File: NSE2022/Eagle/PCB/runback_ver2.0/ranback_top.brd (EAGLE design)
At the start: 100 x 61.3 mm, 25 parts

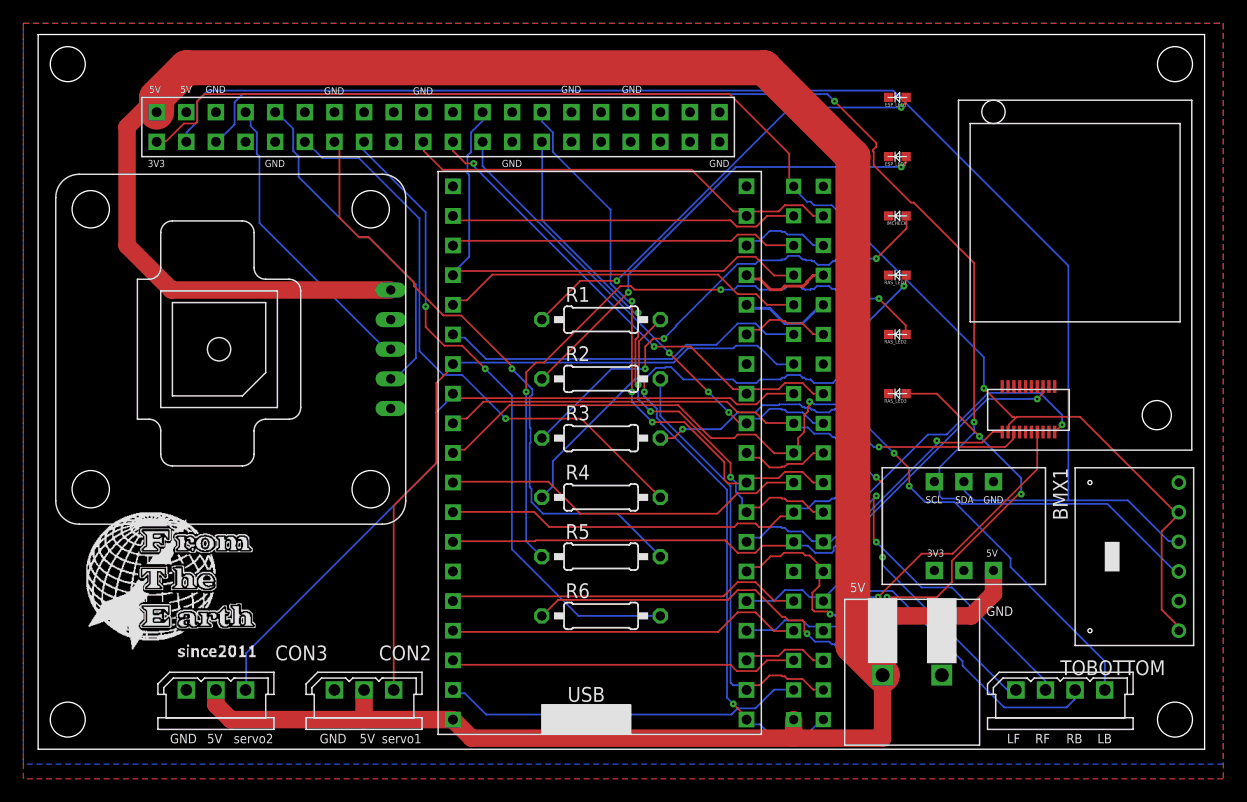
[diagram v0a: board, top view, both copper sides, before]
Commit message: sdf
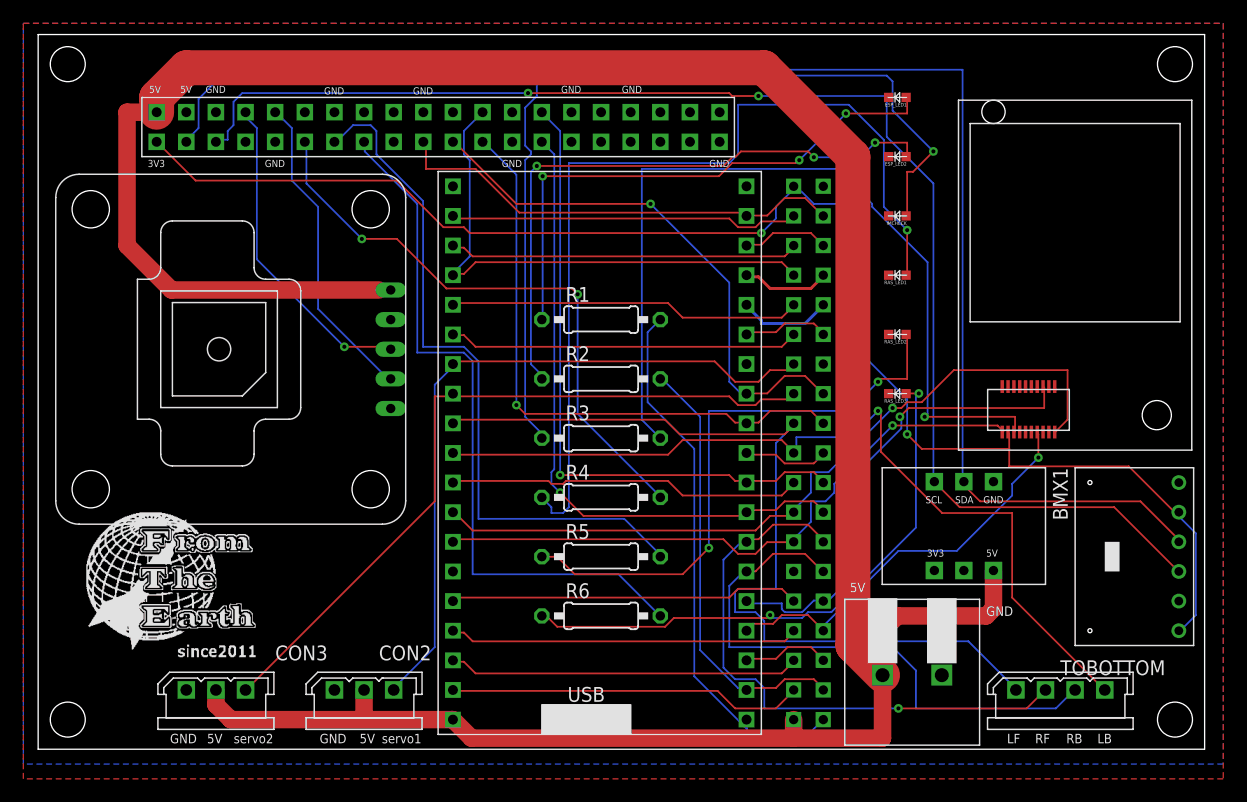
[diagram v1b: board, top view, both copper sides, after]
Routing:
- net LED3: track 34.1 -> 74.2 mm, vias 2 -> 1
- net N$3: track 41.6 -> 77.5 mm, vias 3 -> 1
- net N$4: track 43.9 -> 78.2 mm
- net N$6: track 65.1 -> 49.1 mm, vias 4 -> 2
- net MD_LF: track 63.4 -> 78.4 mm, vias 2 -> 0
- net N$2: track 40.3 -> 53.2 mm, vias 2 -> 3
- net MD_RF: track 38.2 -> 50.8 mm, vias 2 -> 1
- net RP_SCK: track 41.5 -> 51.6 mm, vias 3 -> 1
- net MD_RB: track 40.8 -> 49.4 mm, vias 1 -> 0
- net LED5: track 52.5 -> 60.4 mm, vias 1 -> 0
- net N$1: track 39.4 -> 47.2 mm, vias 2 -> 3
- net RP_TX: track 48.5 -> 55.3 mm, vias 4 -> 1
- net +3V3: track 121.4 -> 128.2 mm, vias 1 -> 2
- net RP_RX: track 49.2 -> 55.4 mm, vias 3 -> 1
- net IM_BUSY: track 60.3 -> 66.0 mm
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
